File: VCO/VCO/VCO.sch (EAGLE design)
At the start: 17 parts, among them IC1 AD711N, IC2 AD711N, T1 BC337, T2 BC337

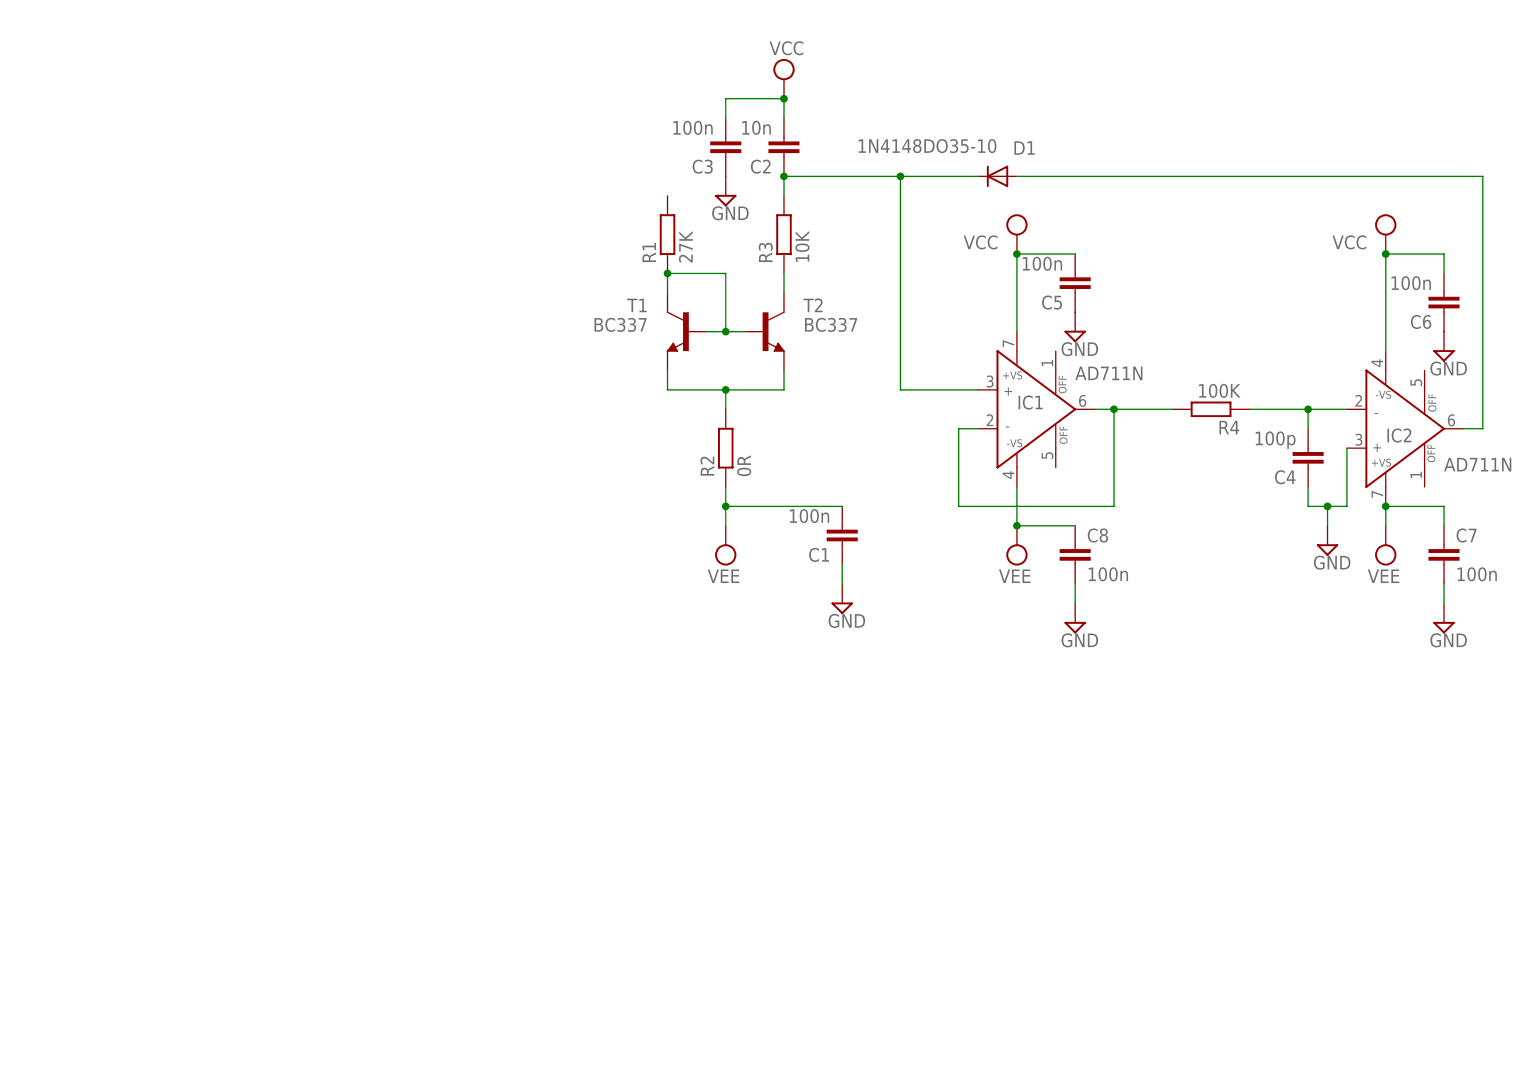
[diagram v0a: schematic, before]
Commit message: Update schematic
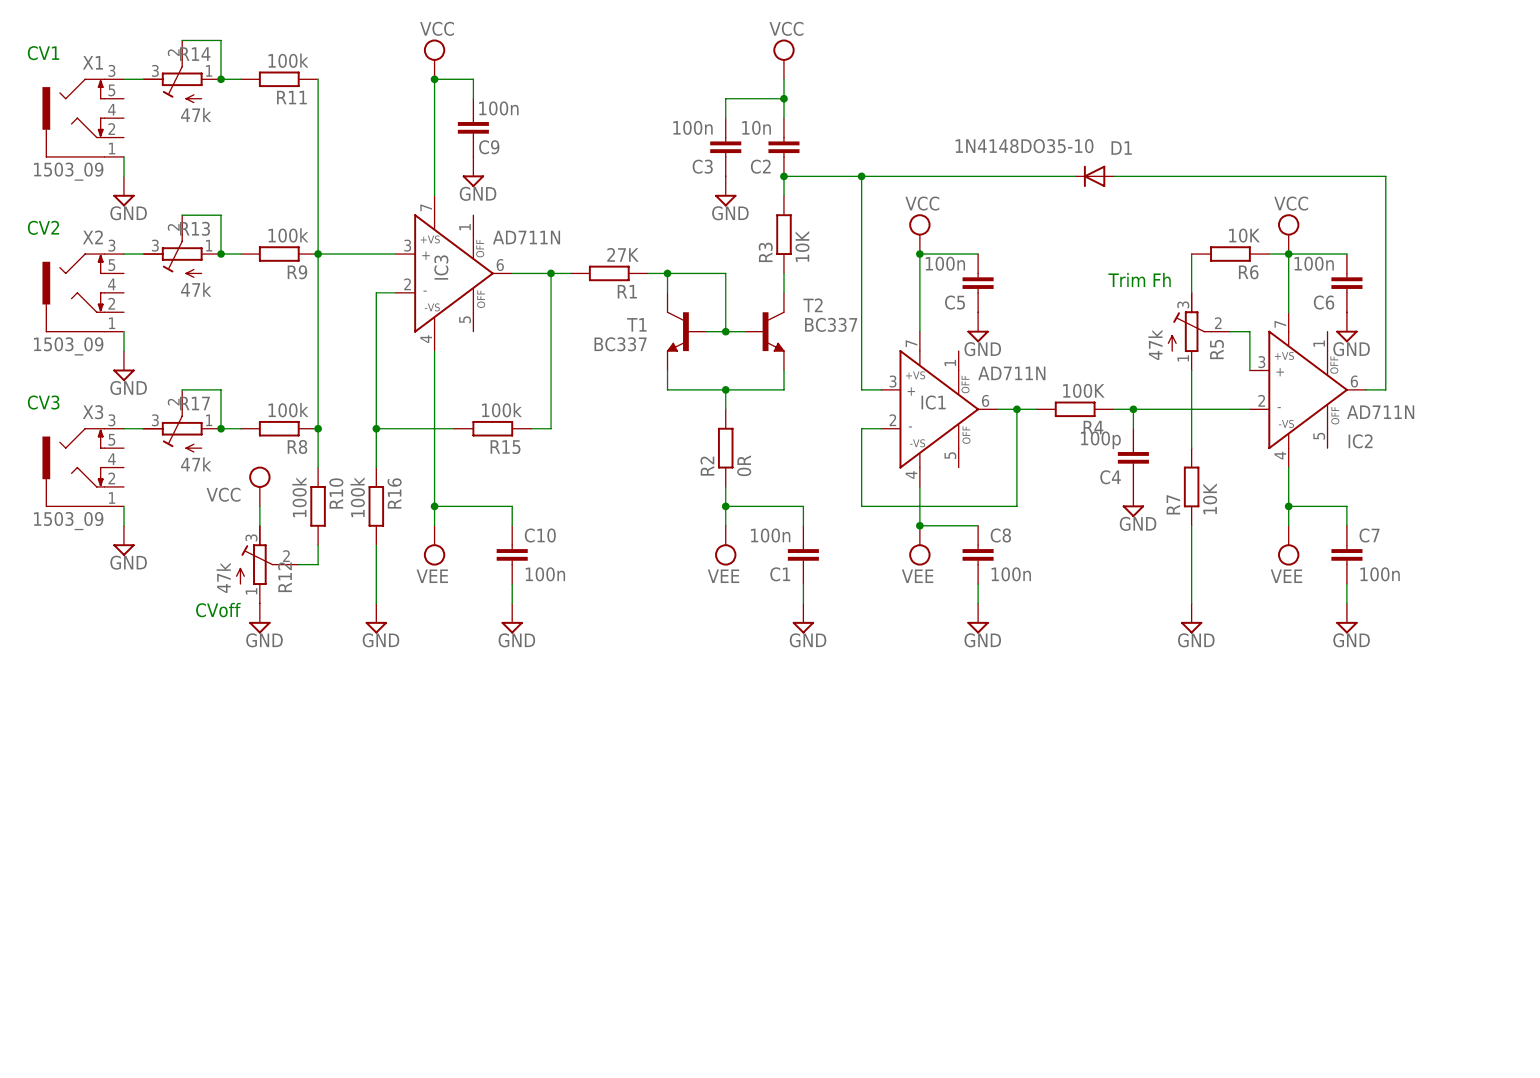
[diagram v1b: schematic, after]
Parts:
- added C10, C9: 100n, capacitor-wima:C5/2.5
- added IC3: AD711N, analog-devices:AD711N
- added R10, R11, R15, R16, R8, R9: 100k, eagle-ltspice:R0207/10
- added R12, R13, R14, R17, R5: 47k, rcl:R-TRIMM64W
- added R6, R7: 10K, eagle-ltspice:R0207/10
- added X1, X2, X3: 1503_09, con-lumberg:1503_09
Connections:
- new net N$10: R10.2, R12.S
- new net N$11: R5.E, R6.2
- new net N$12: R14.E, X1.3
- new net N$13: IC3.IN+, R10.1, R11.1, R8.1, R9.1
- new net N$14: R17.E, X3.3
- new net N$15: R11.2, R14.A, R14.S
- new net N$16: R13.A, R13.S, R9.2
- new net N$17: R13.E, X2.3
- new net N$18: IC3.OUT, R1.2, R15.1
- new net N$19: R17.A, R17.S, R8.2
- new net N$20: IC3.IN-, R15.2, R16.1
- new net N$6: IC2.IN+, R5.S
- new net N$9: R5.A, R7.2
- net GND: now also C10.2, C9.1, R12.A, R16.2, R7.1, X1.1, X2.1, X3.1; no longer IC2.IN+
- net VCC: now also C9.2, IC2.+VS, IC3.+VS, R12.E, R6.1; no longer IC2.-VS
- net VEE: now also C10.1, IC2.-VS, IC3.-VS; no longer IC2.+VS
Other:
- note added: "CV1"
- note added: "CV2"
- note added: "CV3"
- note added: "CVoff"
- note added: "Trim Fh"
- moved on the sheet: C1, C4, C5, C6, C7, C8, D1, IC1, IC2, R1, R4

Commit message: Schematic update
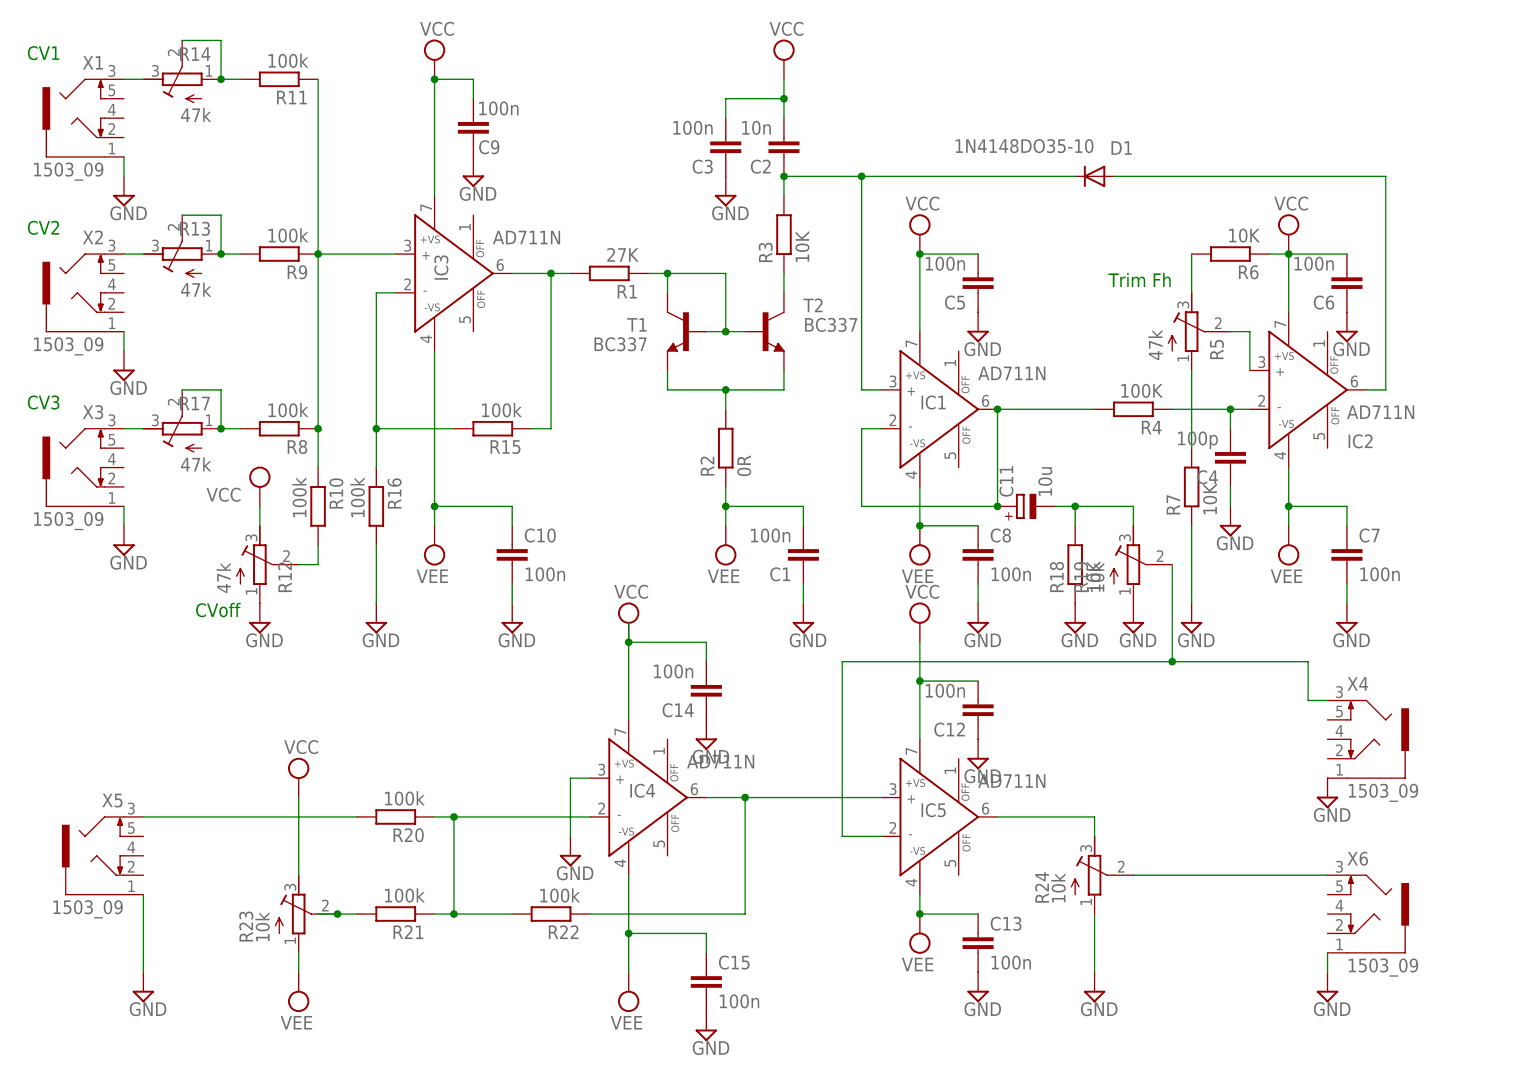
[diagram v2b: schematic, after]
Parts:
- added C11: 10u, rcl:CPOL-EUE2.5-7
- added C12, C13, C14, C15: 100n, capacitor-wima:C5/2.5
- added IC4, IC5: AD711N, analog-devices:AD711N
- added R18: 10K, eagle-ltspice:R0207/10
- added R19, R23, R24: 10k, resistor:R-TRIMM3339P
- added R20, R21, R22: 100k, eagle-ltspice:R0207/10
- added X4, X5, X6: 1503_09, con-lumberg:1503_09
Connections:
- new net N$21: IC5.IN-, R19.S, X4.3
- new net N$22: IC5.OUT, R24.E
- new net N$23: R24.S, X6.3
- new net N$24: IC4.IN-, R20.1, R21.1, R22.2
- new net N$25: C11.-, R18.2, R19.E
- new net N$27: R20.2, X5.3
- new net N$28: R21.2, R23.S
- new net N$29: IC4.OUT, IC5.IN+, R22.1
- net GND: now also C12.1, C13.2, C14.1, C15.2, IC4.IN+, R18.1, R19.A, R24.A, X4.1, X5.1, X6.1
- net N$8: now also C11.+
- net VCC: now also C12.2, C14.2, IC4.+VS, IC5.+VS, R23.E
- net VEE: now also C13.1, C15.1, IC4.-VS, IC5.-VS, R23.A
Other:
- moved on the sheet: C4, R4
